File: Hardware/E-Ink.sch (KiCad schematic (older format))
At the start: 0 parts

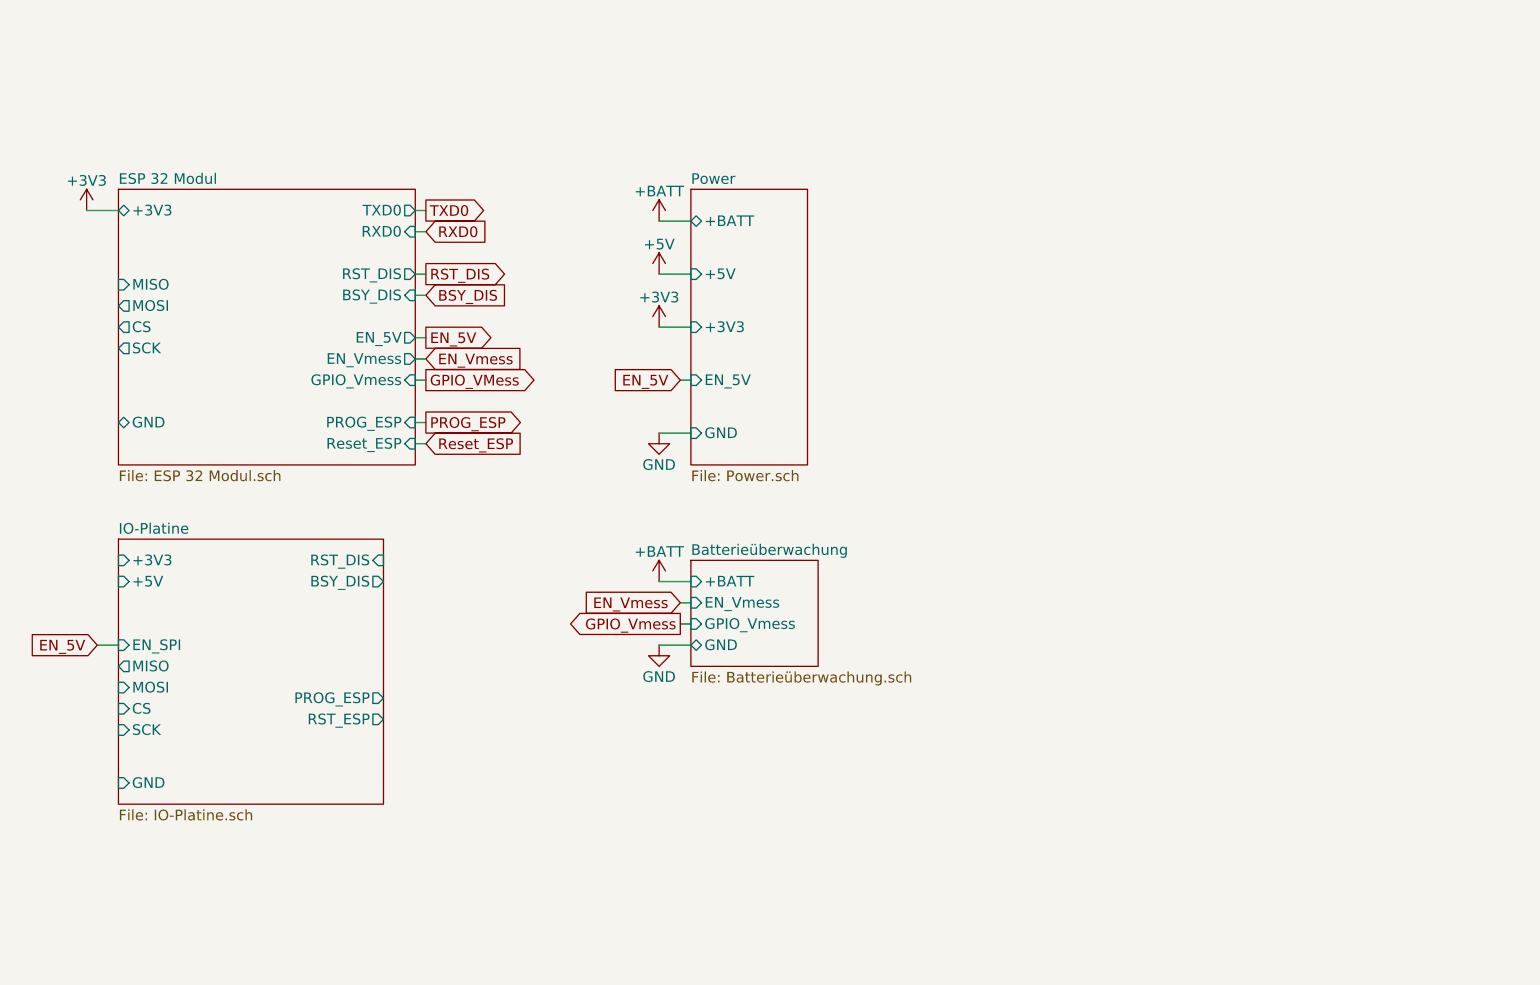
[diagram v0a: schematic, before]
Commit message: Martin ist unförmig
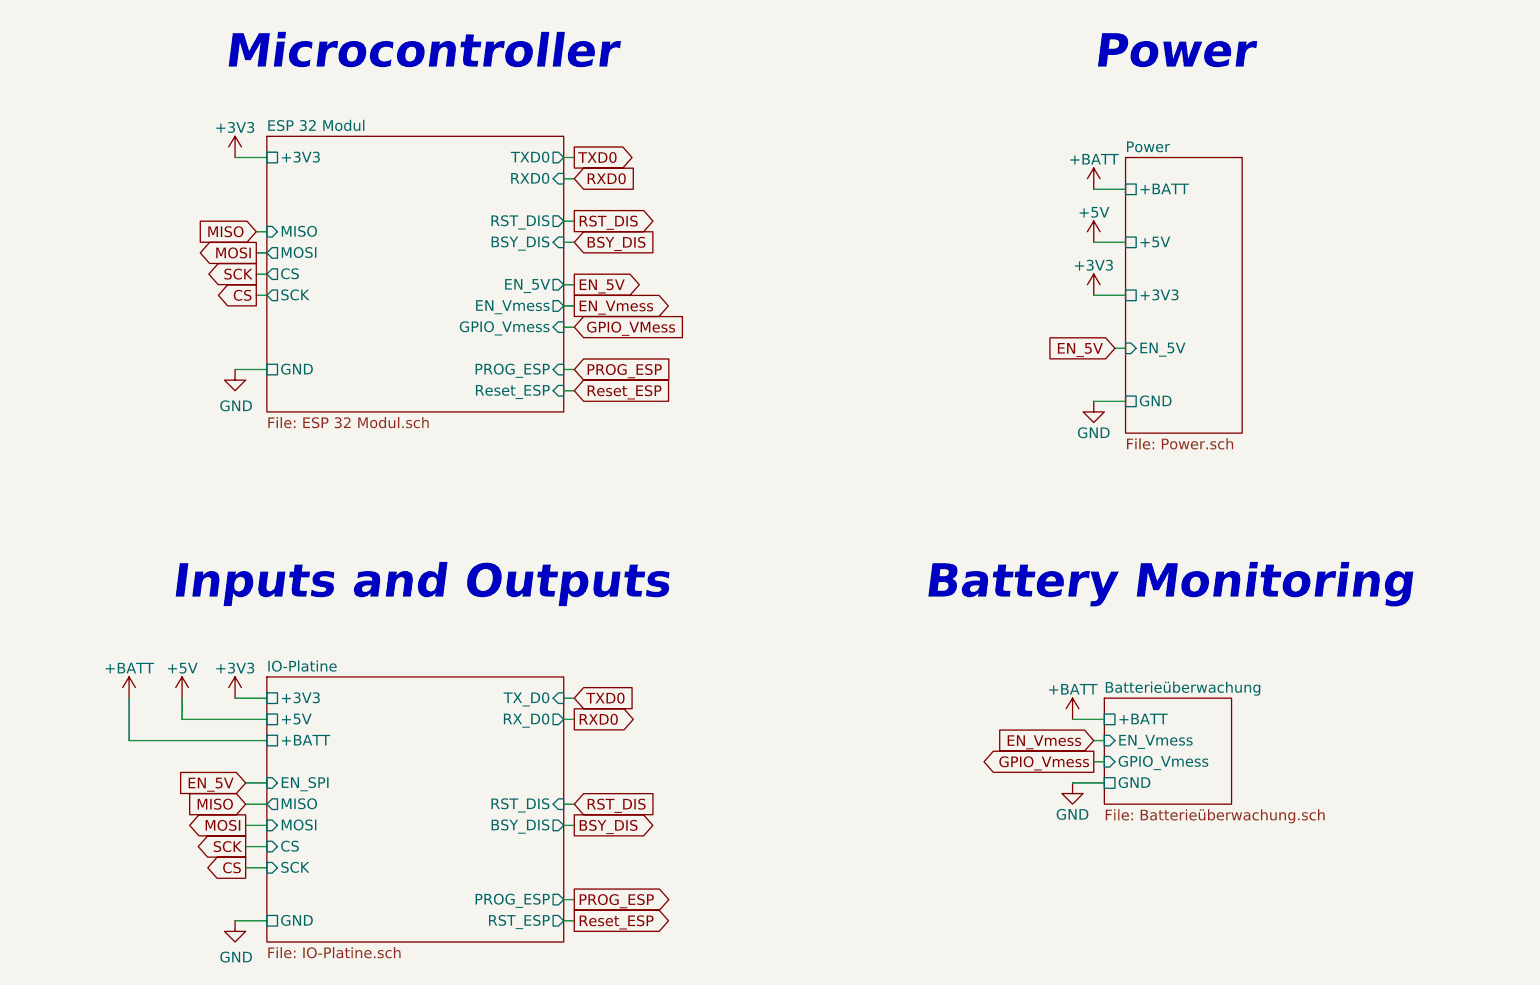
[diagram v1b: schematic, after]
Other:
- note added: "Battery Monitoring"
- note added: "Inputs and Outputs"
- note added: "Microcontroller"
- note added: "Power"

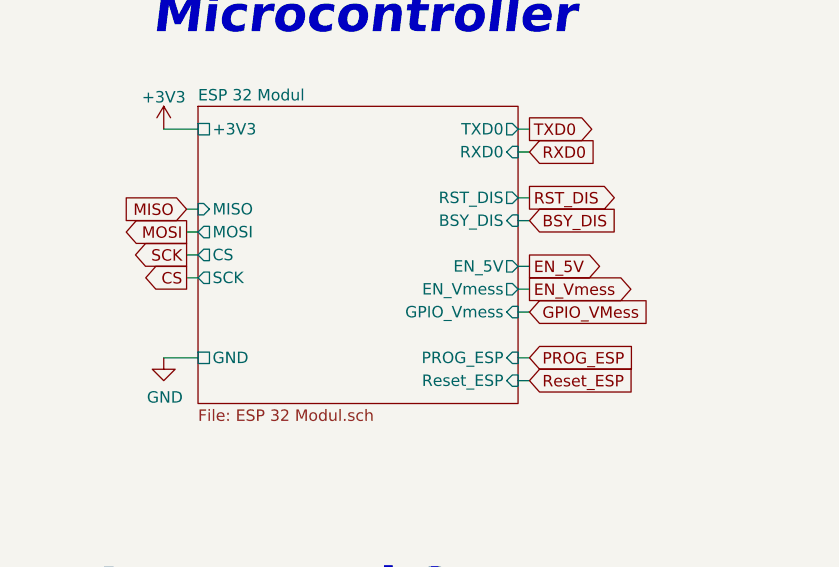
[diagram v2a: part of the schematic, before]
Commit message: save work at arges, finished layout and routing
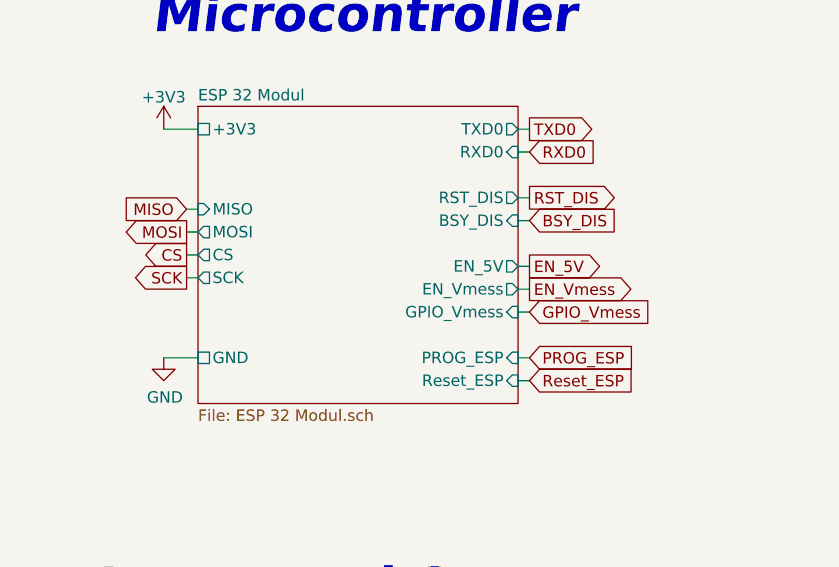
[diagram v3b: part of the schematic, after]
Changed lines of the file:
@@
 EESchema Schematic File Version 4
 LIBS:E-Ink-cache
-EELAYER 29 0
+EELAYER 30 0
 EELAYER END
 $Descr A4 11693 8268
@@
 	4350 3050 4400 3050
 Text GLabel 4400 3150 2    50   Input ~ 0
-GPIO_VMess
+GPIO_Vmess
 Wire Wire Line
 	4400 3150 4350 3150
@@
 Text GLabel 2900 2800 0    50   Output ~ 0
 MOSI
+Text GLabel 2900 3000 0    50   Output ~ 0
+SCK
 Text GLabel 2900 2900 0    50   Output ~ 0
-SCK
-Text GLabel 2900 3000 0    50   Output ~ 0
 CS
 Text GLabel 2850 5400 0    50   Input ~ 0

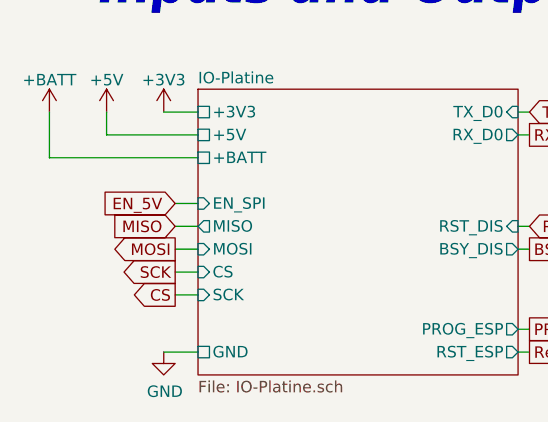
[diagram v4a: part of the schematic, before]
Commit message: Save work at Arges
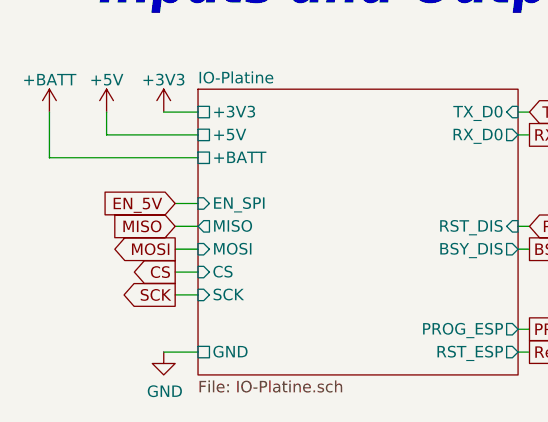
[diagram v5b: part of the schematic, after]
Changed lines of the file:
@@
 EESchema Schematic File Version 4
+LIBS:E-Ink-cache
 EELAYER 30 0
 EELAYER END
@@
 Text GLabel 2850 5500 0    50   Output ~ 0
 MOSI
+Text GLabel 2850 5700 0    50   Output ~ 0
+SCK
 Text GLabel 2850 5600 0    50   Output ~ 0
-SCK
-Text GLabel 2850 5700 0    50   Output ~ 0
 CS
 Wire Wire Line
